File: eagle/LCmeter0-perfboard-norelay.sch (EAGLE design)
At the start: 25 parts, among them IC1 PIC16F876A-X/SP, K2 DS2Y, Q1 20MHz, Q2 BC548, SW1 SPST, SW2 DPDT

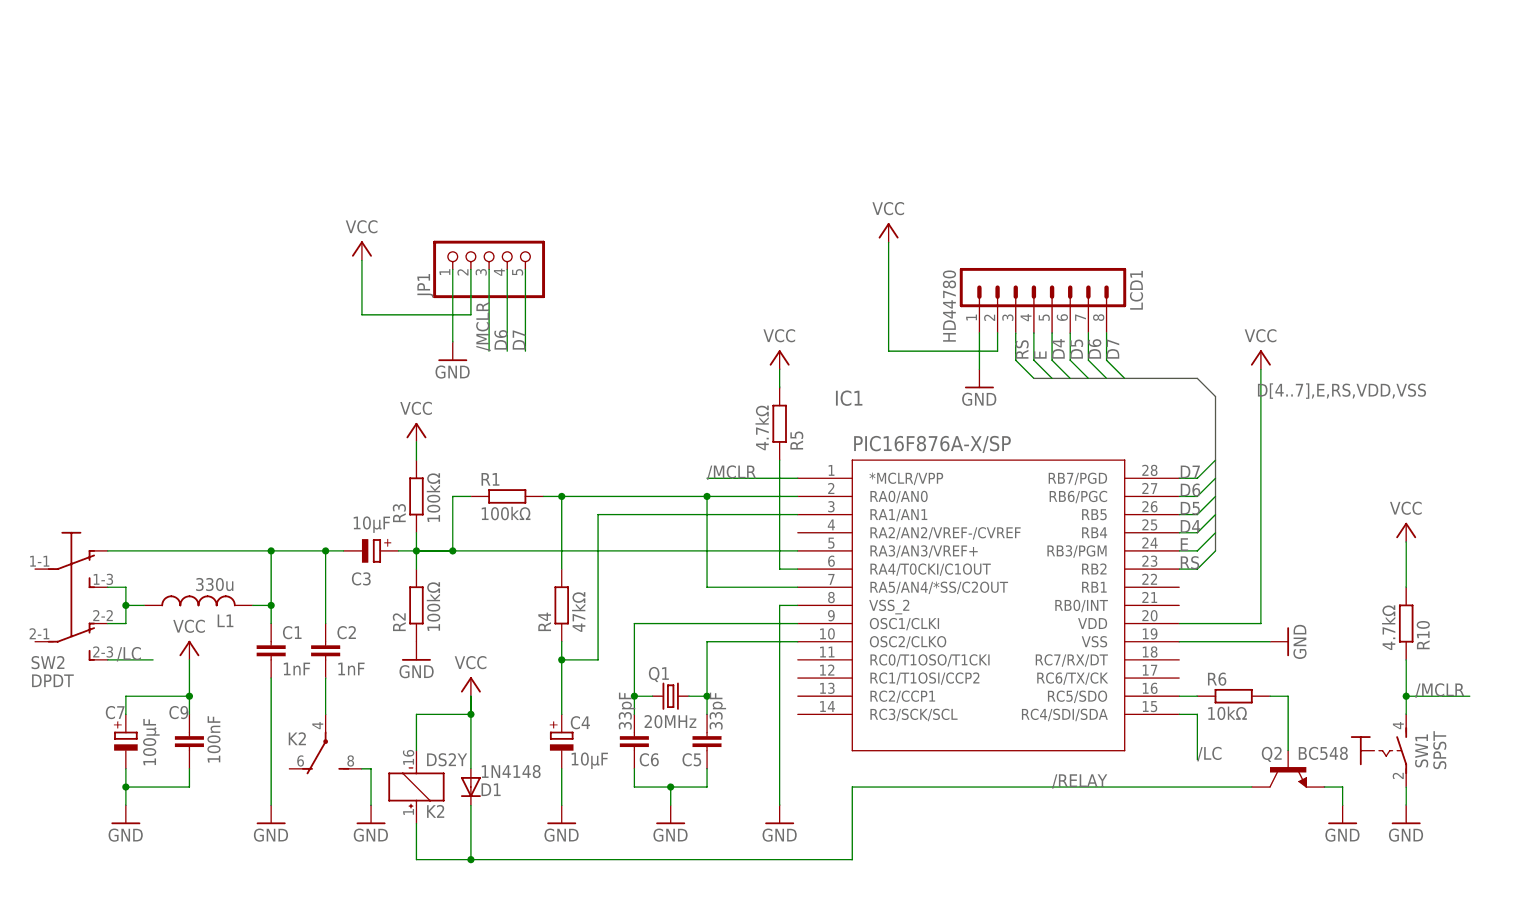
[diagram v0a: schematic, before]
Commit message: ...
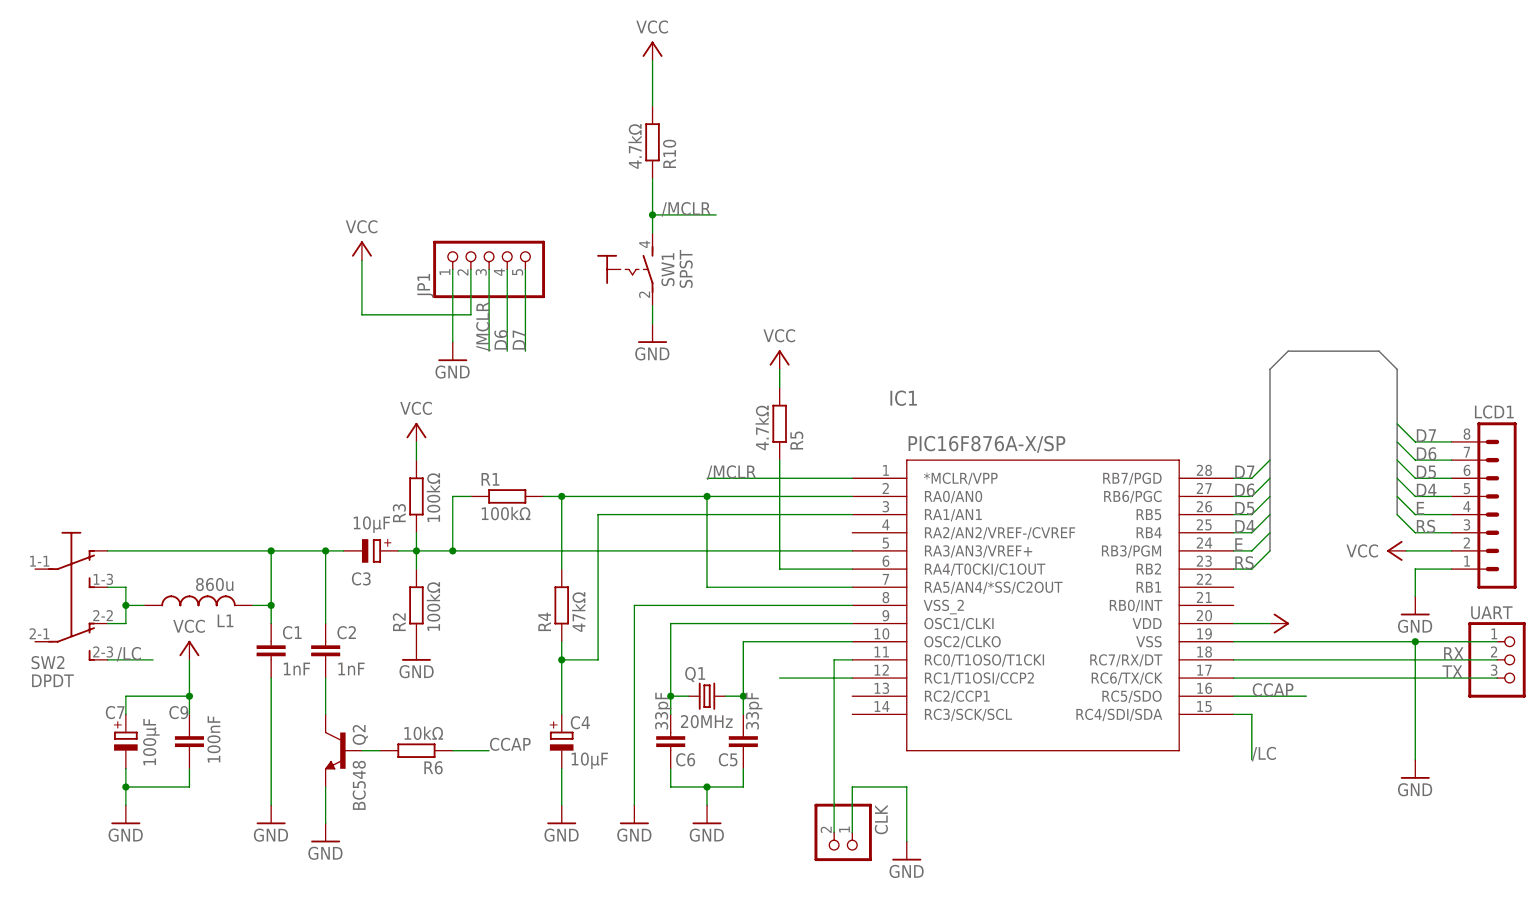
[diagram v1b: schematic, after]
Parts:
- removed D1: 1N4148, diode:1N4148DO35-7
- removed K2: DS2Y, relay:DS2Y-S-DC5V
- added CLK: (no value), pinhead:PINHD-1X2
- added UART: (no value), pinhead:PINHD-1X3
- C3, C4: device rcl:CPOL-EUE2.5-5 -> rcl:CPOL-EUE5-4
- L1: value 330u -> 860u
- R1: device rcl:R-EU_0207/10 -> rcl:R-EU_0204/7
- R10: device resistor:R-EU_0207/10 -> resistor:R-EU_0204/2V
- R2, R3: device resistor:R-EU_0204/2V -> resistor:R-EU_0204/7
- R6: device resistor:R-EU_0204/7 -> resistor:R-EU_0207/10
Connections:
- net RC5 renamed CCAP
- removed net /RELAY: D1.C, K21.+, Q2.C
- new net N$1: CLK.2, IC1.RC0/T1OSO/T1CKI
- new net N$3: IC1.RC1/T1OSI/CCP2
- new net RX: IC1.RC7/RX/DT, UART.2
- new net TX: IC1.RC6/TX/CK, UART.3
- net C2_CON: now also Q2.C; no longer K22.P
- net GND: now also CLK.1, UART.1; no longer K22.S
- net VCC: no longer D1.A, K21.-
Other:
- moved on the sheet: C5, C6, IC1, LCD1, Q1, Q2, R10, R6, SW1

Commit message: ...
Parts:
- IC1: device lc-meter:PIC16F876A-X/SP -> mcu:PIC16F876A-X/SP
- SW1: device lc-meter:PB-5-2 -> mcu:PB-5-2
- SW2: device lc-meter:S-DPDT -> mcu:S-DPDT
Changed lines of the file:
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@@
 </classes>
 <parts>
-<part name="IC1" library="lc-meter" deviceset="PIC16F876A-X/SP" device=""/>
+<part name="IC1" library="mcu" deviceset="PIC16F876A-X/SP" device=""/>
 <part name="R1" library="rcl" deviceset="R-EU_" device="0204/7" value="100kΩ"/>
 <part name="R2" library="resistor" deviceset="R-EU_" device="0204/7" value="100kΩ"/>
@@
 <part name="R5" library="resistor" deviceset="R-EU_" device="0204/7" value="4.7kΩ"/>
 <part name="P+5" library="supply1" deviceset="VCC" device=""/>
-<part name="SW2" library="lc-meter" deviceset="S-DPDT" device="" value="DPDT"/>
-<part name="SW1" library="lc-meter" deviceset="PB-5-2" device="" value="SPST"/>
+<part name="SW2" library="mcu" deviceset="S-DPDT" device="" value="DPDT"/>
+<part name="SW1" library="mcu" deviceset="PB-5-2" device="" value="SPST"/>
 <part name="P+6" library="supply1" deviceset="VCC" device=""/>
 <part name="Q2" library="transistor-npn" deviceset="BC548*" device=""/>

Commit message: ...
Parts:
- Q1: device crystal:CRYSTALHC49S -> q:CRYSTALHC49S
- Q2: device transistor-npn:BC548 -> t:BC548
- R10, R4: device resistor:R-EU_0204/2V -> r:R-EU_0204/2V
- R2, R3, R5: device resistor:R-EU_0204/7 -> r:R-EU_0204/7
- R6: device resistor:R-EU_0207/10 -> r:R-EU_0207/10
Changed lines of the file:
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@@
 <part name="IC1" library="mcu" deviceset="PIC16F876A-X/SP" device=""/>
 <part name="R1" library="rcl" deviceset="R-EU_" device="0204/7" value="100kΩ"/>
-<part name="R2" library="resistor" deviceset="R-EU_" device="0204/7" value="100kΩ"/>
-<part name="R3" library="resistor" deviceset="R-EU_" device="0204/7" value="100kΩ"/>
-<part name="R4" library="resistor" deviceset="R-EU_" device="0204/2V" value="47kΩ"/>
-<part name="R10" library="resistor" deviceset="R-EU_" device="0204/2V" value="4.7kΩ"/>
+<part name="R2" library="r" deviceset="R-EU_" device="0204/7" value="100kΩ"/>
+<part name="R3" library="r" deviceset="R-EU_" device="0204/7" value="100kΩ"/>
+<part name="R4" library="r" deviceset="R-EU_" device="0204/2V" value="47kΩ"/>
+<part name="R10" library="r" deviceset="R-EU_" device="0204/2V" value="4.7kΩ"/>
 <part name="C1" library="rcl" deviceset="C-EU" device="050-024X044" value="1nF"/>
 <part name="C2" library="rcl" deviceset="C-EU" device="050-024X044" value="1nF"/>
@@
 <part name="GND7" library="supply1" deviceset="GND" device=""/>
 <part name="L1" library="rcl" deviceset="L-US" device="0204/5" value="860u"/>
-<part name="Q1" library="crystal" deviceset="CRYSTAL" device="HC49S" value="20MHz"/>
+<part name="Q1" library="q" deviceset="CRYSTAL" device="HC49S" value="20MHz"/>
 <part name="P+1" library="supply1" deviceset="VCC" device=""/>
 <part name="GND11" library="supply1" deviceset="GND" device=""/>
@@
 <part name="P+4" library="supply1" deviceset="VCC" device=""/>
 <part name="GND12" library="supply1" deviceset="GND" device=""/>
-<part name="R5" library="resistor" deviceset="R-EU_" device="0204/7" value="4.7kΩ"/>
+<part name="R5" library="r" deviceset="R-EU_" device="0204/7" value="4.7kΩ"/>
 <part name="P+5" library="supply1" deviceset="VCC" device=""/>
 <part name="SW2" library="mcu" deviceset="S-DPDT" device="" value="DPDT"/>
 <part name="SW1" library="mcu" deviceset="PB-5-2" device="" value="SPST"/>
 <part name="P+6" library="supply1" deviceset="VCC" device=""/>
-<part name="Q2" library="transistor-npn" deviceset="BC548*" device=""/>
+<part name="Q2" library="t" deviceset="BC548*" device=""/>
 <part name="GND8" library="supply1" deviceset="GND" device=""/>
-<part name="R6" library="resistor" deviceset="R-EU_" device="0207/10" value="10kΩ"/>
+<part name="R6" library="r" deviceset="R-EU_" device="0207/10" value="10kΩ"/>
 <part name="LCD1" library="con-lstb" deviceset="MA08-1" device="" value="HD44780"/>
 <part name="GND1" library="supply1" deviceset="GND" device=""/>
